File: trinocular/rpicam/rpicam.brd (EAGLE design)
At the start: 90 x 90 mm, 9 parts, among them IC1 MEGA8-AI

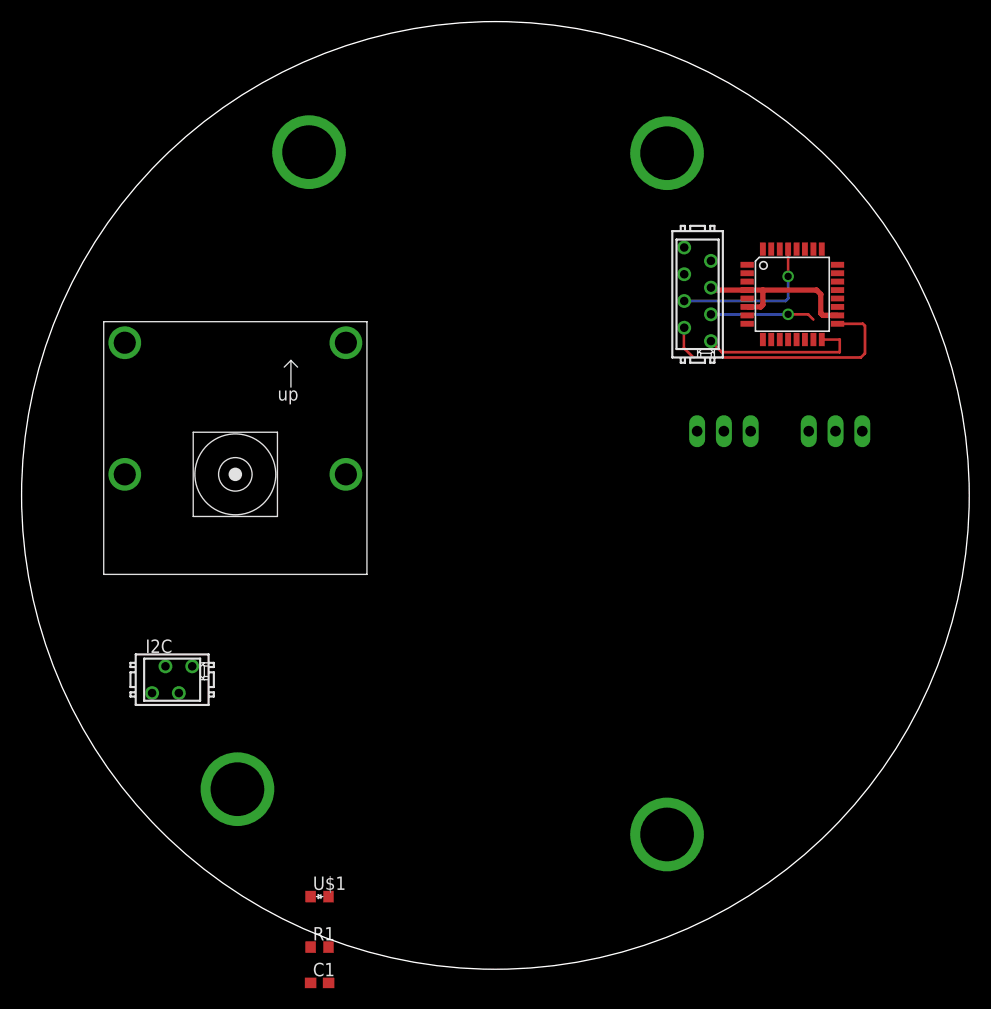
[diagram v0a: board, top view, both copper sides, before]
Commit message: 03-12-13 20:52
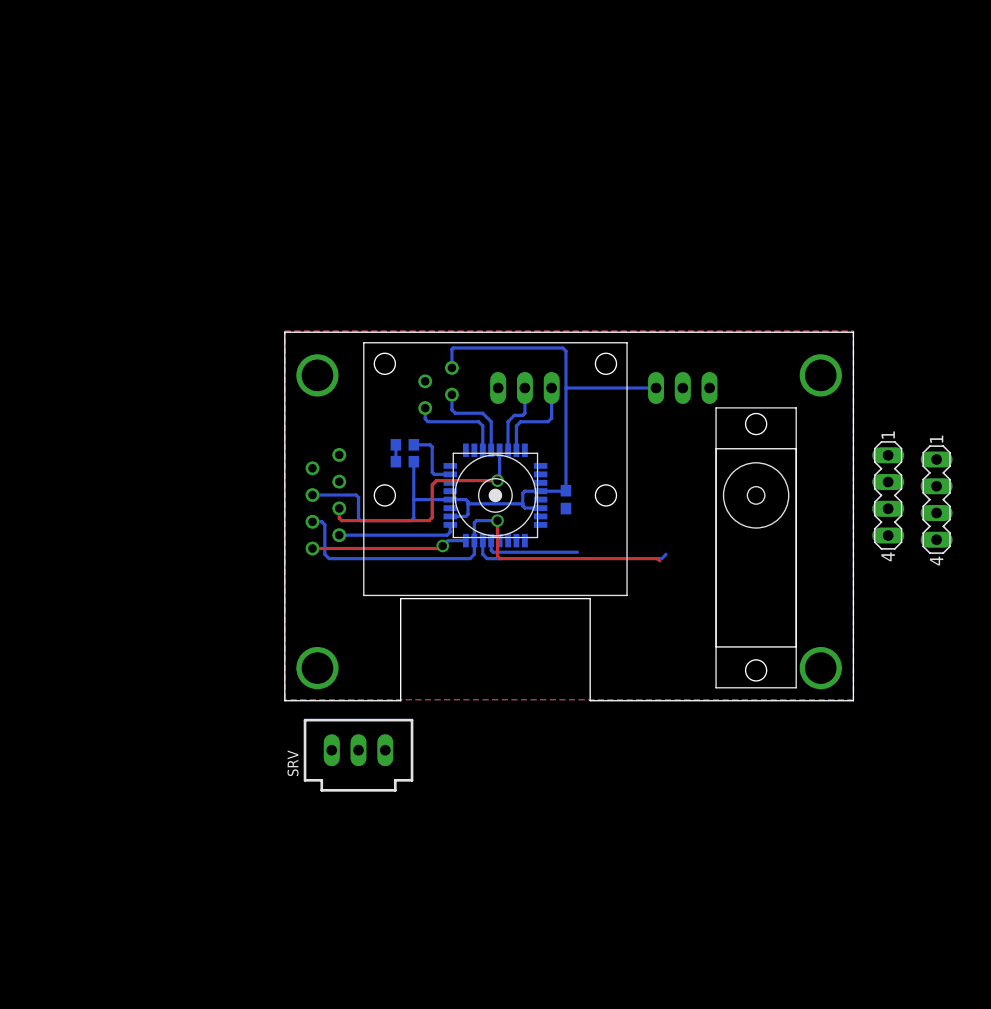
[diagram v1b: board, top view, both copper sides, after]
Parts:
- added LEDD#1, LEDD#2: (no value), con-lstb:MA04-1
- added SRV: power, con-molex:70543-03
- added U$3: (no value), servos:HS-35HD
- U$2: value RPICAM -> (none)
- moved C1 51.5 mm to (6.70, -0.40), flipped to the bottom, turned to 90 degrees
- moved R1 48.4 mm to (-8.60, 4.80), flipped to the bottom
- moved U$1 42.1 mm to (-8.60, 3.20), flipped to the bottom
- moved ISP 40.4 mm to (-16.1, -0.60), flipped to the bottom
- moved I2C 37.5 mm to (-5.40, 10.2), flipped to the bottom, turned to 270 degrees
- moved IC1 34.1 mm to (0.00, 0.00), flipped to the bottom
- moved U$2 24.8 mm to (0.00, 0.00)
- moved UART 19.3 mm to (2.80, 10.2), turned to 180 degrees
- moved PWR 15.1 mm to (17.8, 10.2), turned to 180 degrees
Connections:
- removed net N$3: I2C.3
- removed net N$5: I2C.4
- removed net N$9: R1.2, U$1.1
- new net SCL: I2C.2, IC1.28
- new net SDA: I2C.1, IC1.27
- net +12V: now also LEDD#1.3, LEDD#2.3
- net +5V: now also I2C.4, LEDD#1.1, LEDD#2.1, U$1.1; no longer U$1.2
- net GND: now also I2C.3, LEDD#1.4, LEDD#2.4, SRV.3
- net LED1_CTRL: now also LEDD#1.2
- net LED2_CTRL: now also LEDD#2.2
- net MOSI/SRV_CTRL: now also SRV.1
- net N$1: now also R1.2, U$1.2; no longer I2C.1
- net N$2: now also SRV.2; no longer I2C.2
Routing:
- net +5V: track 17.1 -> 72.4 mm
- net MOSI/SRV_CTRL: track 10.7 -> 42.9 mm
- net LED2_CTRL: track 0.00 -> 19.0 mm
- net SCK: track 25.0 -> 11.3 mm
- net LED1_CTRL: track 0.00 -> 9.19 mm
- net SDA: track 0.00 -> 9.08 mm
- net TXD: track 0.00 -> 8.81 mm
- net SCL: track 0.00 -> 8.34 mm
- net RST: track 14.7 -> 22.4 mm
- net RXD: track 0.00 -> 7.04 mm
- net N$4: track 0.00 -> 6.02 mm
- net N$1: track 0.00 -> 1.60 mm
- net MISO: track 15.6 -> 14.9 mm, vias 0 -> 1
- added copper zone on layer 1, net GND
- added copper zone on layer 16, net GND
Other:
- board size 90 x 90 mm -> 54 x 35 mm
